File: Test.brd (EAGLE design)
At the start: 43.2 x 53 mm, 17 parts, among them U1 ESP-WROOM-32

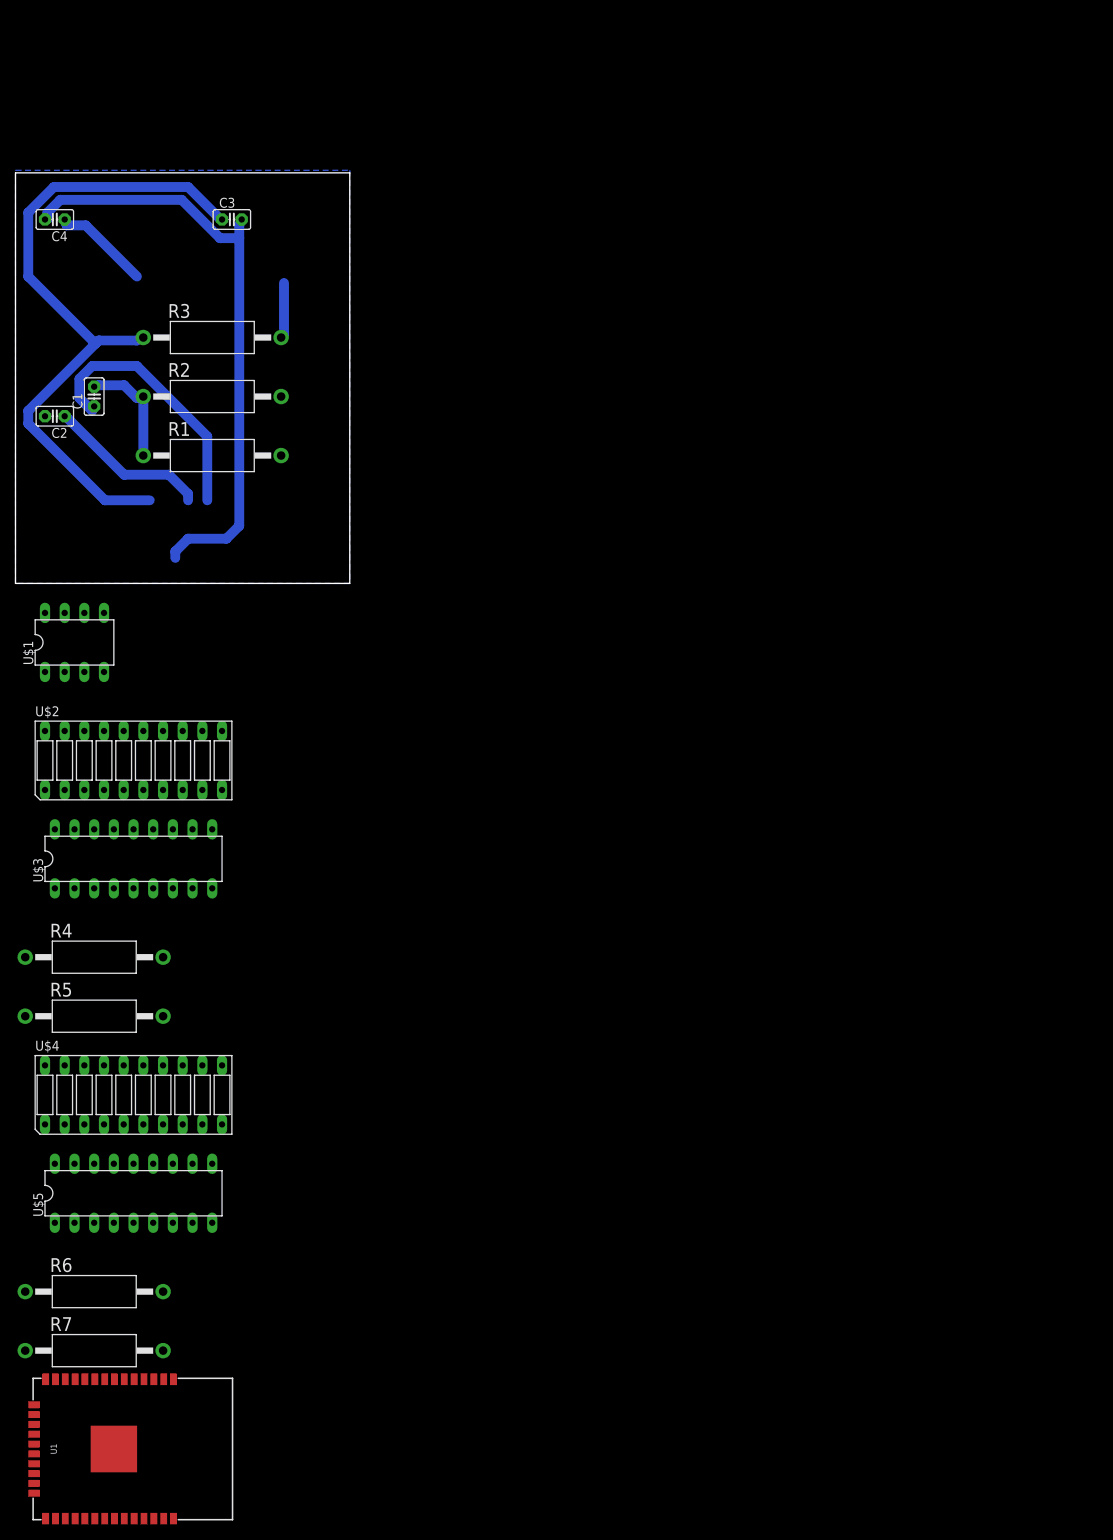
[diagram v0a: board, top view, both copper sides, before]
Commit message: [fix]手直し
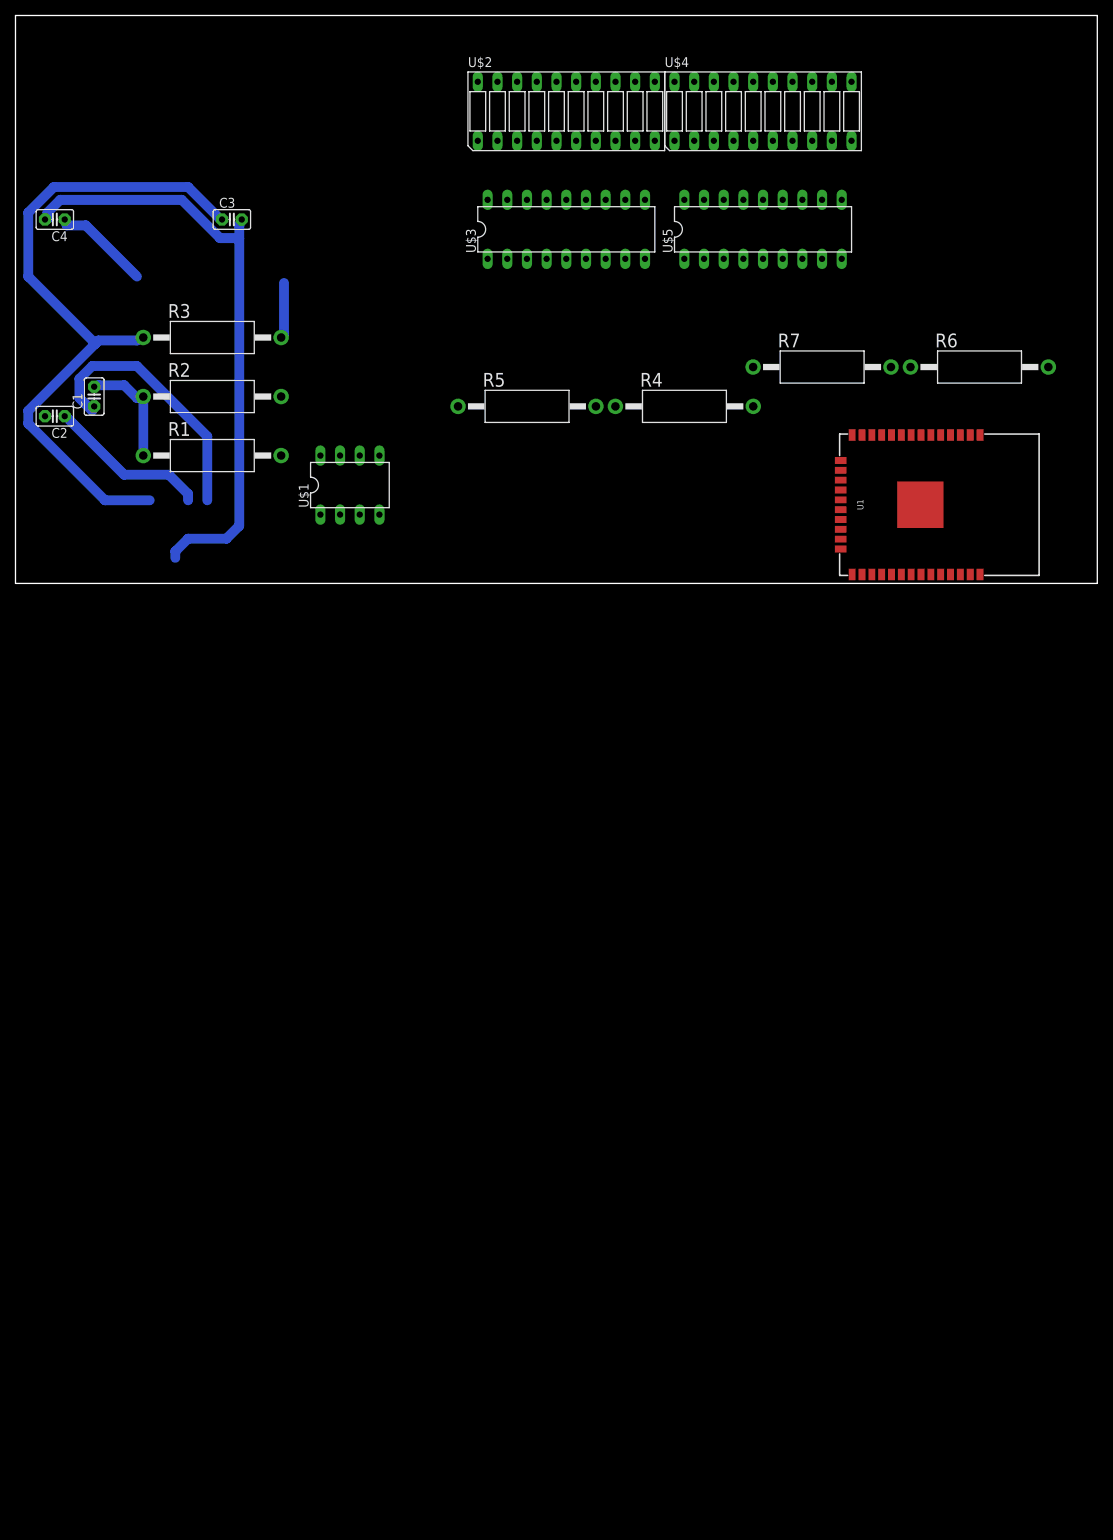
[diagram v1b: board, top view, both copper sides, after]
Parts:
- moved R6 165.3 mm to (124.5, 27.9)
- moved U1 160.3 mm to (116.8, 10.2)
- moved R7 158.0 mm to (104.1, 27.9)
- moved U$4 150.8 mm to (96.5, 61.0)
- moved U$5 148.6 mm to (96.5, 45.7)
- moved R4 104.2 mm to (86.4, 22.9)
- moved U$2 100.7 mm to (71.1, 61.0)
- moved U$3 98.6 mm to (71.1, 45.7)
- moved R5 96.6 mm to (66.0, 22.9)
- moved U$1 41.0 mm to (43.2, 12.7)
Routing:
- removed copper zone on layer 16, net N$6
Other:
- board size 43.2 x 53 mm -> 139.7 x 73.3 mm
